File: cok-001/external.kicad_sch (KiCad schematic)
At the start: 69 parts, among them J3208 凸, J3209 ATA Power, J3219 for Multi_Card_Board, J3221 IMSA-9637S-60Y801, Q3201 DTC144E

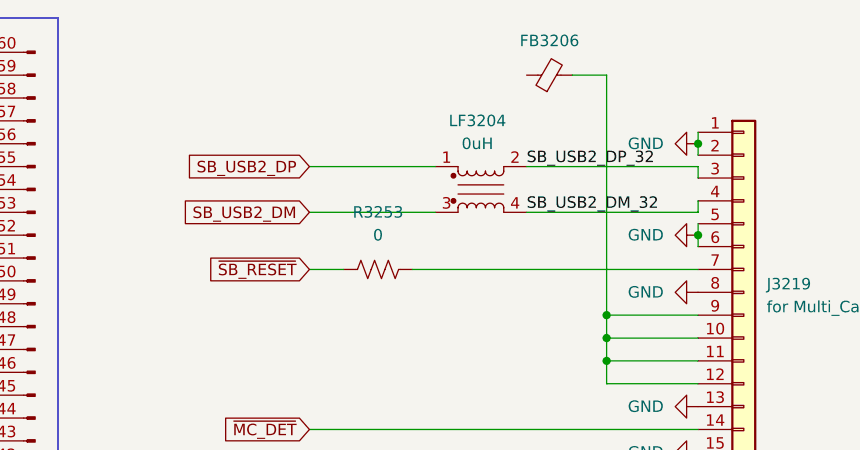
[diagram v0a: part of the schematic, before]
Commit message: lf
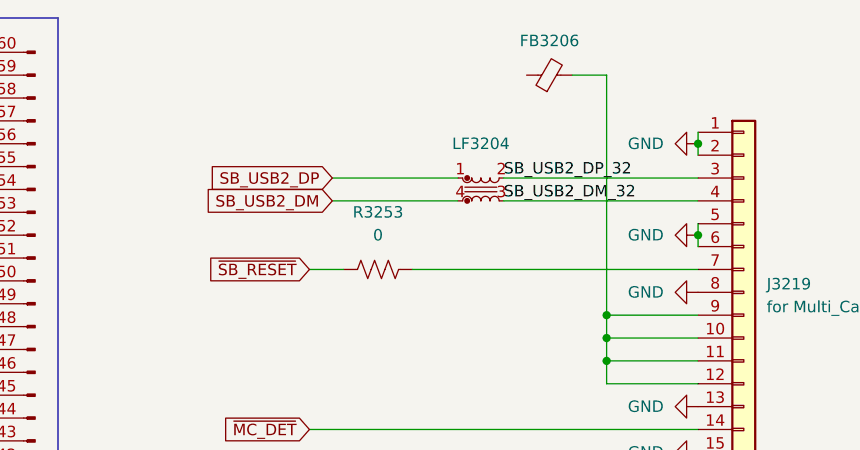
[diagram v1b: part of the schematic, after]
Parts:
- LF3204: value 0uH -> L_Iron_Coupled_Small_1243; symbol Device:Filter_EMI_LL -> Device:L_Iron_Coupled_Small_1243
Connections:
- net SB_USB2_DM: now also LF3204.4; no longer LF3204.3
- net SB_USB2_DM_32: now also LF3204.3; no longer LF3204.4
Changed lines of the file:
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@@
 	(wire
 		(pts
-			(xy 213.36 35.56) (xy 213.36 34.29)
-		)
-		(stroke
-			(width 0)
-			(type default)
-		)
-	)
-	(wire
-		(pts
 			(xy 127 154.94) (xy 134.62 154.94)
 		)
@@
 	(wire
 		(pts
-			(xy 194.31 35.56) (xy 213.36 35.56)
+			(xy 191.77 34.29) (xy 213.36 34.29)
 		)
 		(stroke
@@
 	(wire
 		(pts
-			(xy 170.18 30.48) (xy 184.15 30.48)
+			(xy 172.72 31.75) (xy 186.69 31.75)
 		)
 		(stroke
@@
 	(wire
 		(pts
-			(xy 213.36 30.48) (xy 213.36 31.75)
-		)
-		(stroke
-			(width 0)
-			(type default)
-		)
-	)
-	(wire
-		(pts
 			(xy 81.28 76.2) (xy 101.6 76.2)
 		)
@@
 	(wire
 		(pts
-			(xy 194.31 30.48) (xy 213.36 30.48)
+			(xy 191.77 31.75) (xy 213.36 31.75)
 		)
 		(stroke
@@
 	(wire
 		(pts
-			(xy 170.18 35.56) (xy 184.15 35.56)
+			(xy 172.72 34.29) (xy 186.69 34.29)
 		)
 		(stroke
@@
 	)
 	(label "SB_USB2_DP_32"
-		(at 194.31 30.48 0)
+		(at 191.77 31.75 0)
 		(effects
 			(font
@@
 	)
 	(label "SB_USB2_DM_32"
-		(at 194.31 35.56 0)
+		(at 191.77 34.29 0)
 		(effects
 			(font
@@
 	(global_label "SB_USB2_DP"
 		(shape input)
-		(at 170.18 30.48 180)
+		(at 172.72 31.75 180)
 		(fields_autoplaced yes)
 		(effects
@@
 		)
 		(property "Intersheetrefs" "${INTERSHEET_REFS}"
-			(at 155.2206 30.48 0)
+			(at 157.7606 31.75 0)
 			(hide yes)
 			(show_name no)
@@
 	(global_label "SB_USB2_DM"
 		(shape input)
-		(at 170.18 35.56 180)
+		(at 172.72 34.29 180)
 		(fields_autoplaced yes)
 		(effects
@@
 		)
 		(property "Intersheetrefs" "${INTERSHEET_REFS}"
-			(at 155.0392 35.56 0)
+			(at 157.5792 34.29 0)
 			(hide yes)
 			(show_name no)
@@
 	)
 	(symbol
-		(lib_id "Device:Filter_EMI_LL")
+		(lib_id "Device:L_Iron_Coupled_Small_1243")
 		(at 189.23 33.02 0)
 		(unit 1)
@@
 		(in_pos_files yes)
 		(dnp no)
-		(fields_autoplaced yes)
 		(property "Reference" "LF3204"
-			(at 188.849 25.4 0)
+			(at 189.23 27.94 0)
 			(show_name no)
 			(do_not_autoplace no)
@@
 			)
 		)
-		(property "Value" "0uH"
-			(at 188.849 27.94 0)
+		(property "Value" "L_Iron_Coupled_Small_1243"
+			(at 189.23 29.21 0)
+			(hide yes)
 			(show_name no)
 			(do_not_autoplace no)
@@
 		)
 		(property "Footprint" ""
-			(at 189.23 32.004 0)
+			(at 189.23 33.02 0)
 			(hide yes)
 			(show_name no)
@@
 		)
 		(property "Datasheet" ""
-			(at 189.23 32.004 0)
+			(at 189.23 33.02 0)
 			(hide yes)
 			(show_name no)
@@
 			)
 		)
-		(property "Description" "EMI 2-inductor filter"
+		(property "Description" "Coupled inductor with iron core, small symbol"
 			(at 189.23 33.02 0)
 			(hide yes)
